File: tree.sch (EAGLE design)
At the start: 16 parts, among them U1 ATTINY13A-PU

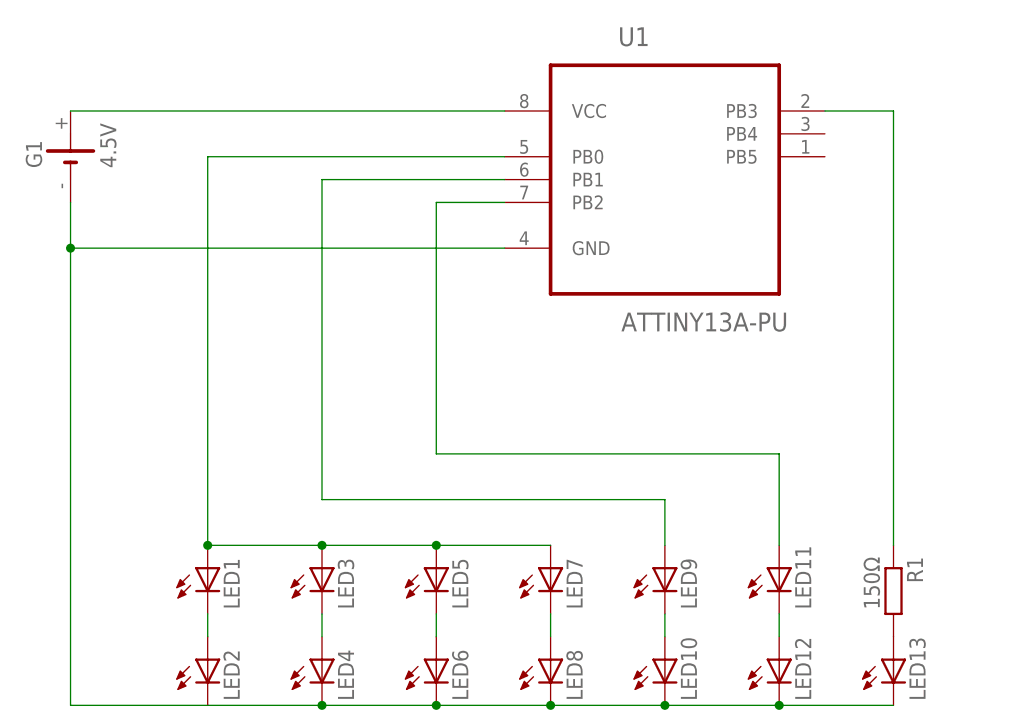
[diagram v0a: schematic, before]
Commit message: v1.0
That’s it. (I’m pretty sure)
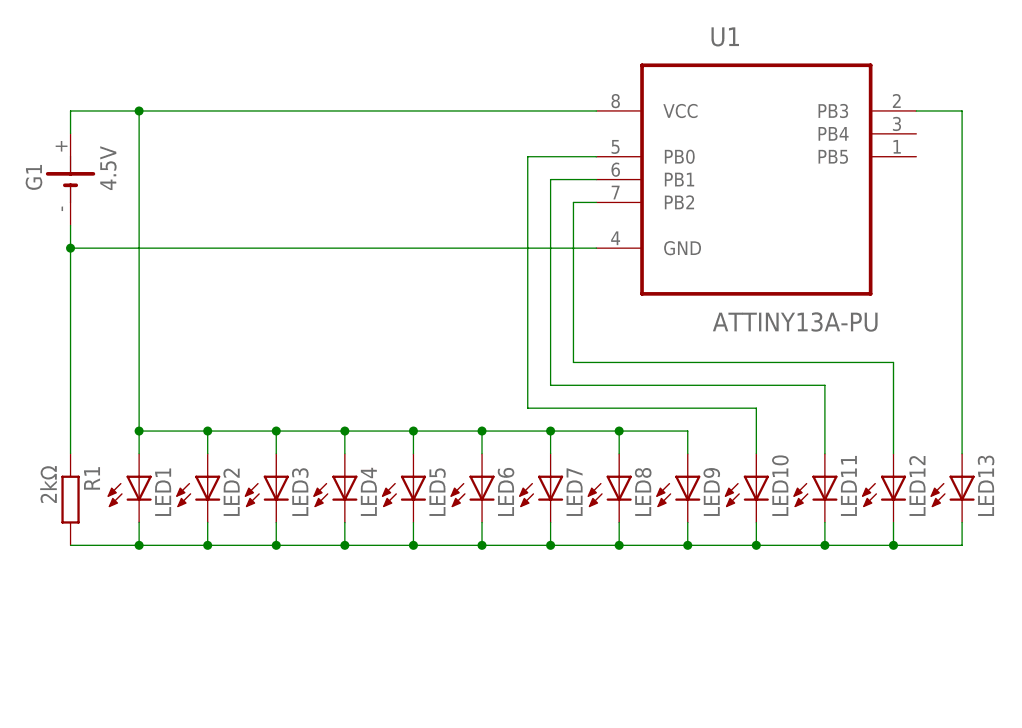
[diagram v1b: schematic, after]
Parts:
- R1: value 150Ω -> 2kΩ
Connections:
- removed net N$13: LED13.A, R1.2
- removed net N$14: LED10.C, LED12.C, LED13.C, LED2.C, LED4.C, LED6.C, LED8.C
- removed net N$15: G1.+, U1.VCC
- removed net N$16: LED1.A, LED3.A, LED5.A, LED7.A, U1.PB0
- removed net N$22: LED9.A, U1.PB1
- removed net N$24: LED11.A, U1.PB2
- removed net N$8: R1.1, U1.PB3
- net N$1: now also G1.+, LED1.A, LED3.A, LED4.A, LED5.A, LED6.A, LED7.A, LED8.A, LED9.A, U1.VCC; no longer LED1.C
- net N$2: now also LED1.C, LED10.C, LED11.C, LED12.C, LED13.C, LED2.C, LED4.C, LED5.C, LED6.C, LED7.C, LED8.C, LED9.C, R1.2; no longer LED4.A
- net N$3: now also LED13.A, U1.PB3; no longer LED5.C, LED6.A
- net N$4: now also LED12.A, U1.PB2; no longer LED7.C, LED8.A
- net N$5: now also LED11.A, U1.PB1; no longer LED10.A, LED9.C
- net N$6: now also LED10.A, U1.PB0; no longer LED11.C, LED12.A
- net N$7: now also R1.1
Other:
- moved on the sheet: G1, LED1, LED10, LED11, LED12, LED13, LED2, LED3, LED4, LED5, LED6, LED7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
